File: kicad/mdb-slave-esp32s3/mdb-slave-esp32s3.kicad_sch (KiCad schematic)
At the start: 36 parts, among them J1 Conn_02x09_Odd_Even, J2 MDB_Connector, P1 USB_C_Plug_USB2.0, SW1 Reset, SW2 Boot, U1 ESP32-S3, U2 LM317_SOT-223, U4 PC817, U5 PC817, Y1 Crystal

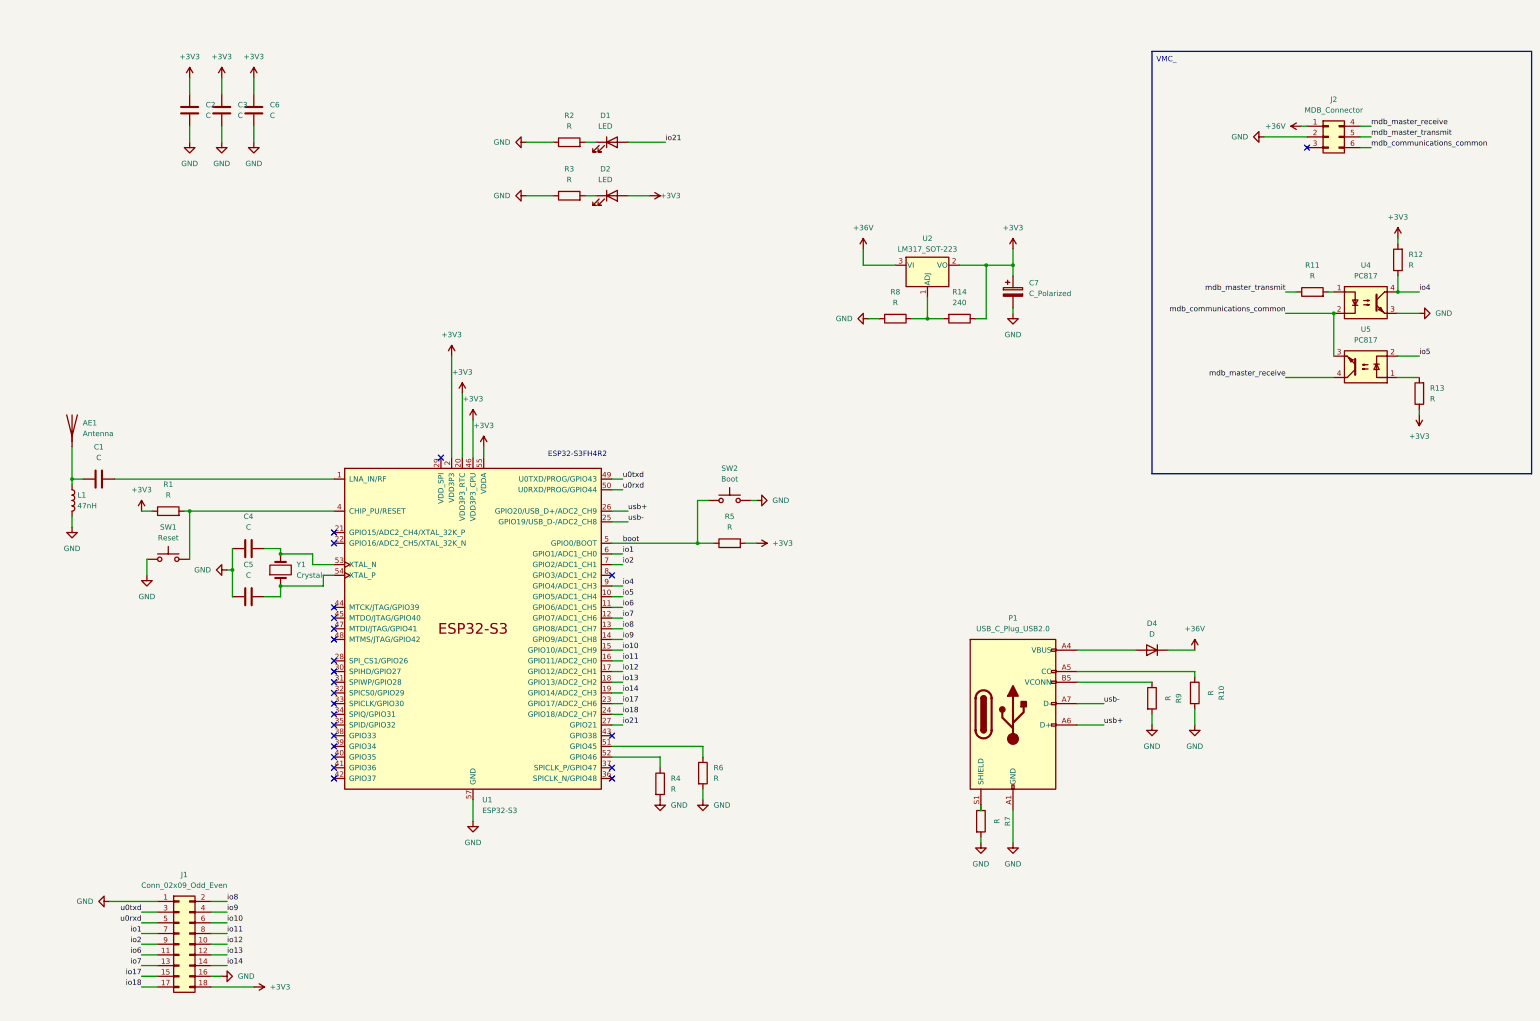
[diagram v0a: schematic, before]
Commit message: refacting
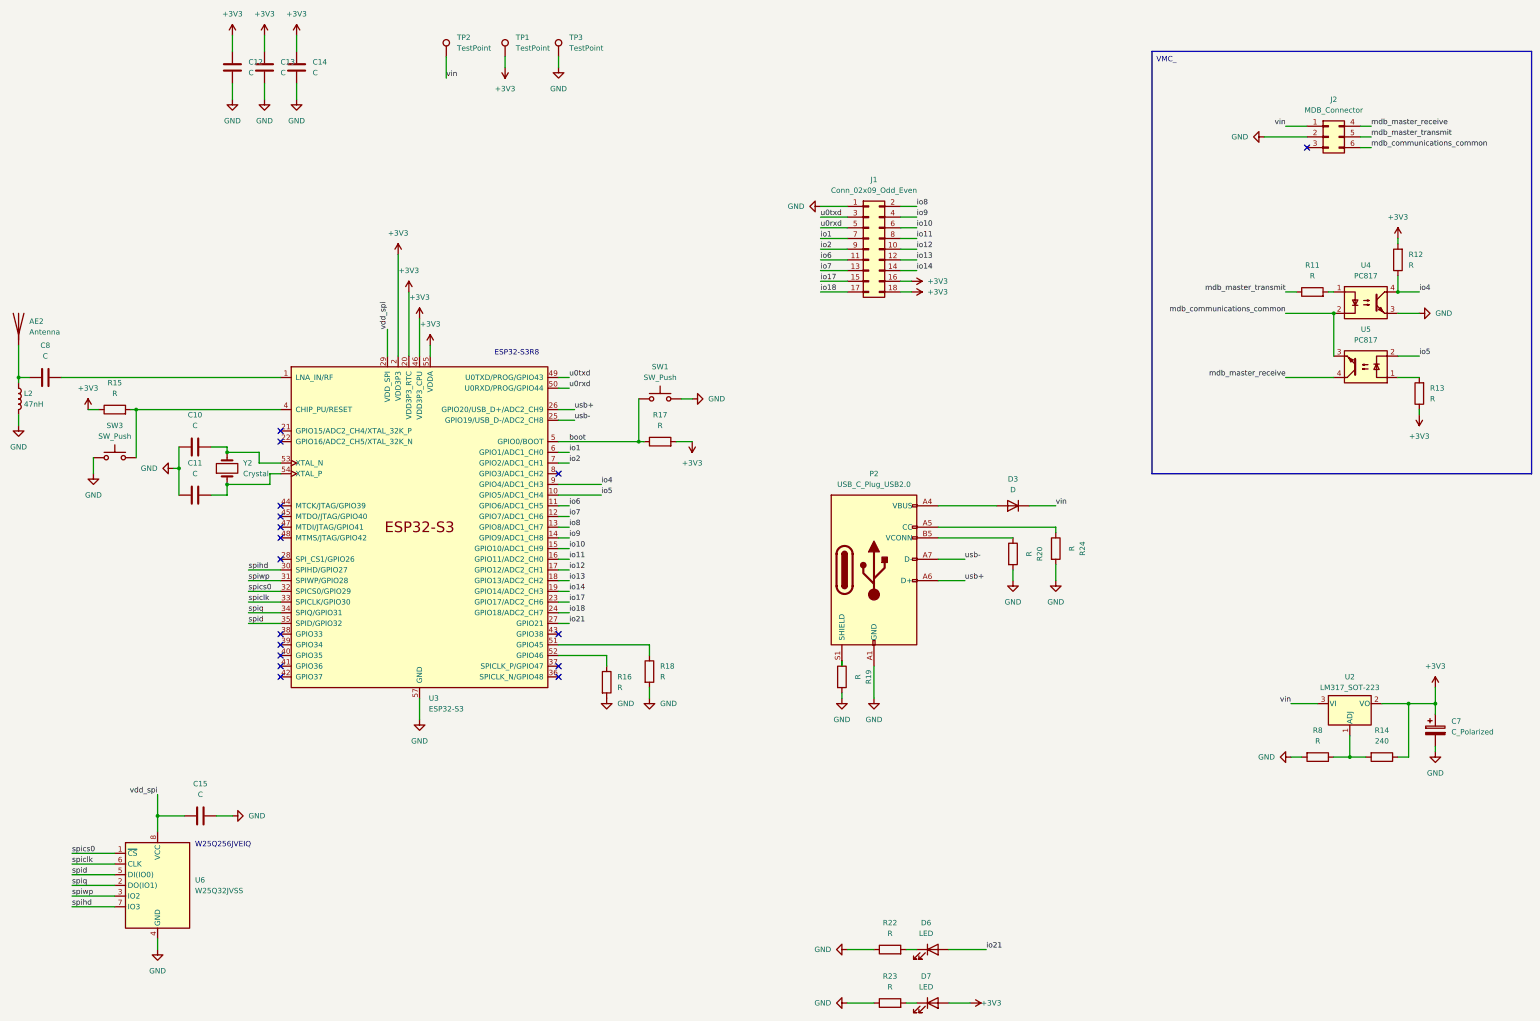
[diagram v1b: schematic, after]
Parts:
- removed AE1: Antenna, RF_Antenna:Texas_SWRA117D_2.4GHz_Right, symbol Device:Antenna
- removed C1, C2, C3, C4, C5, C6: C, Capacitor_SMD:C_0603_1608Metric, symbol Device:C
- removed D1, D2: LED, LED_SMD:LED_0603_1608Metric, symbol Device:LED
- removed D4: D, Diode_SMD:D_SOD-123, symbol Device:D
- removed L1: 47nH, Inductor_SMD:L_0603_1608Metric, symbol Device:L
- removed P1: USB_C_Plug_USB2.0, Connector_USB:USB_C_Receptacle_G-Switch_GT-USB-7010ASV, symbol Connector:USB_C_Plug_USB2.0
- removed R1, R10, R2, R3, R4, R5, R6, R7, R9: R, Resistor_SMD:R_0603_1608Metric, symbol Device:R
- removed SW2: Boot, Button_Switch_SMD:SW_Tactile_SPST_NO_Straight_CK_PTS636Sx25SMTRLFS, symbol Switch:SW_Push
- removed U1: ESP32-S3, Package_DFN_QFN:QFN-56-1EP_7x7mm_P0.4mm_EP5.6x5.6mm, symbol PCM_Espressif:ESP32-S3
- removed Y1: Crystal, Crystal:Crystal_HC49-4H_Vertical, symbol Device:Crystal
- added AE2: Antenna, RF_Antenna:Texas_SWRA117D_2.4GHz_Right, symbol Device:Antenna
- added C10, C11, C12, C13, C14, C15, C8: C, Capacitor_SMD:C_0603_1608Metric, symbol Device:C
- added D3: D, Diode_SMD:D_SOD-123, symbol Device:D
- added D6, D7: LED, LED_SMD:LED_0603_1608Metric, symbol Device:LED
- added L2: 47nH, Inductor_SMD:L_0603_1608Metric, symbol Device:L
- added P2: USB_C_Plug_USB2.0, Connector_USB:USB_C_Receptacle_G-Switch_GT-USB-7010ASV, symbol Connector:USB_C_Plug_USB2.0
- added R15, R16, R17, R18, R19, R20, R22, R23, R24: R, Resistor_SMD:R_0603_1608Metric, symbol Device:R
- added SW3: SW_Push, Button_Switch_SMD:SW_Tactile_SPST_NO_Straight_CK_PTS636Sx25SMTRLFS, symbol Switch:SW_Push
- added TP1, TP2, TP3: TestPoint, TestPoint:TestPoint_Pad_D1.0mm, symbol Connector:TestPoint
- added U3: ESP32-S3, Package_DFN_QFN:QFN-56-1EP_7x7mm_P0.4mm_EP5.6x5.6mm, symbol PCM_Espressif:ESP32-S3
- added U6: W25Q32JVSS, Package_SON:WSON-8-1EP_8x6mm_P1.27mm_EP3.4x4.3mm, symbol Memory_Flash:W25Q32JVSS
- added Y2: Crystal, Crystal:Crystal_HC49-4H_Vertical, symbol Device:Crystal
- SW1: value Reset -> SW_Push
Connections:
- net +3V3: now also J1.16 (Pin_16), C12.2, C13.2, C14.2, D7.2 (A), R15.1, R17.2, TP1.1, U3.2 (VDD3P3), U3.20 (VDD3P3_RTC), U3.3 (VDD3P3), U3.46 (VDD3P3_CPU), U3.55 (VDDA), U3.56 (VDDA)
- net GND: now also SW1.2, C10.1, C11.1, C12.1, C13.1, C14.1, C15.2, L2.2, P2.A1 (GND), P2.A12 (GND), P2.B1 (GND), P2.B12 (GND), R16.2, R18.2, R19.2, R20.2, R22.1, R23.1, R24.2, SW3.1, TP3.1, U3.57 (GND), U6.4 (GND); no longer J1.16 (Pin_16), SW1.1
- net boot: now also SW1.1, R17.1, U3.5 (GPIO0/BOOT)
- net io1: now also U3.6 (GPIO1/ADC1_CH0)
- net io10: now also U3.15 (GPIO10/ADC1_CH9)
- net io11: now also U3.16 (GPIO11/ADC2_CH0)
- net io12: now also U3.17 (GPIO12/ADC2_CH1)
- net io13: now also U3.18 (GPIO13/ADC2_CH2)
- net io14: now also U3.19 (GPIO14/ADC2_CH3)
- net io17: now also U3.23 (GPIO17/ADC2_CH6)
- net io18: now also U3.24 (GPIO18/ADC2_CH7)
- net io2: now also U3.7 (GPIO2/ADC1_CH1)
- net io21: now also D6.2 (A), U3.27 (GPIO21)
- net io4: now also U3.9 (GPIO4/ADC1_CH3)
- net io5: now also U3.10 (GPIO5/ADC1_CH4)
- net io6: now also U3.11 (GPIO6/ADC1_CH5)
- net io7: now also U3.12 (GPIO7/ADC1_CH6)
- net io8: now also U3.13 (GPIO8/ADC1_CH7)
- net io9: now also U3.14 (GPIO9/ADC1_CH8)
- net u0rxd: now also U3.50 (U0RXD/PROG/GPIO44)
- net u0txd: now also U3.49 (U0TXD/PROG/GPIO43)
- net usb+: now also P2.A6 (D+), U3.26 (GPIO20/USB_D+/ADC2_CH9)
- net usb-: now also P2.A7 (D-), U3.25 (GPIO19/USB_D-/ADC2_CH8)
- net +36V renamed vin
- net vin: now also D3.1 (K), TP2.1
- new net: R16.1, U3.52 (GPIO46)
- new net: D7.1 (K), R23.2
- new net: D3.2 (A), P2.A4 (VBUS), P2.A9 (VBUS), P2.B4 (VBUS), P2.B9 (VBUS)
- new net: C10.2, U3.53 (XTAL_N), Y2.2
- new net: C8.2, U3.1 (LNA_IN/RF)
- new net: R15.2, SW3.2, U3.4 (CHIP_PU/RESET)
- new net: R18.1, U3.51 (GPIO45)
- new net: C11.2, U3.54 (XTAL_P), Y2.1
- new net: P2.A5 (CC), R24.1
- new net: P2.B5 (VCONN), R20.1
- new net: P2.S1 (SHIELD), R19.1
- new net: D6.1 (K), R22.2
- new net: AE2.1 (A), C8.1, L2.1
- new net spiclk: U3.33 (SPICLK/GPIO30), U6.6 (CLK)
- new net spics0: U3.32 (SPICS0/GPIO29), U6.1 (~{CS})
- new net spid: U3.35 (SPID/GPIO32), U6.5 (DI(IO0))
- new net spihd: U3.30 (SPIHD/GPIO27), U6.7 (IO3)
- new net spiq: U3.34 (SPIQ/GPIO31), U6.2 (DO(IO1))
- new net spiwp: U3.31 (SPIWP/GPIO28), U6.3 (IO2)
- new net vdd_spi: C15.1, U3.29 (VDD_SPI), U6.8 (VCC)
- no-connect marks 24 -> 17
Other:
- note added: "ESP32-S3R8"
- note added: "W25Q256JVEIQ"
- note removed: "ESP32-S3FH4R2"
- moved on the sheet: C7, R14, R8, U2
